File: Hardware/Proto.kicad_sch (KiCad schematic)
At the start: 6 parts, among them J2 Conn_01x04_Male, J3 Conn_01x02_Male, J4 Conn_01x02_Male, J5 Conn_01x02_Male, J6 Conn_01x02_Male, J9 Conn_01x04_MountingPin

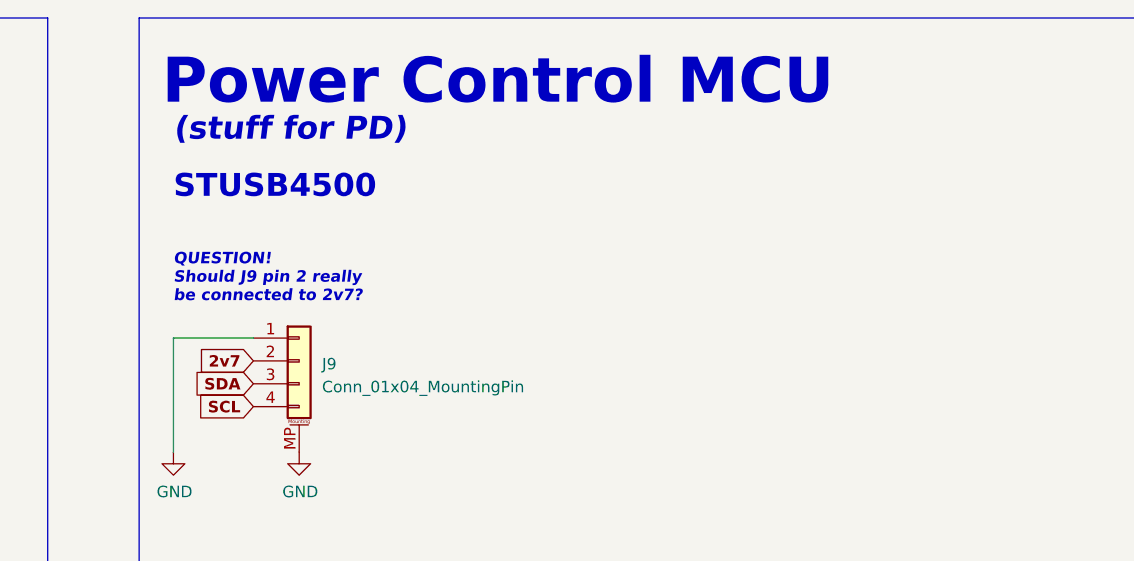
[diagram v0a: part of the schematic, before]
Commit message: .........
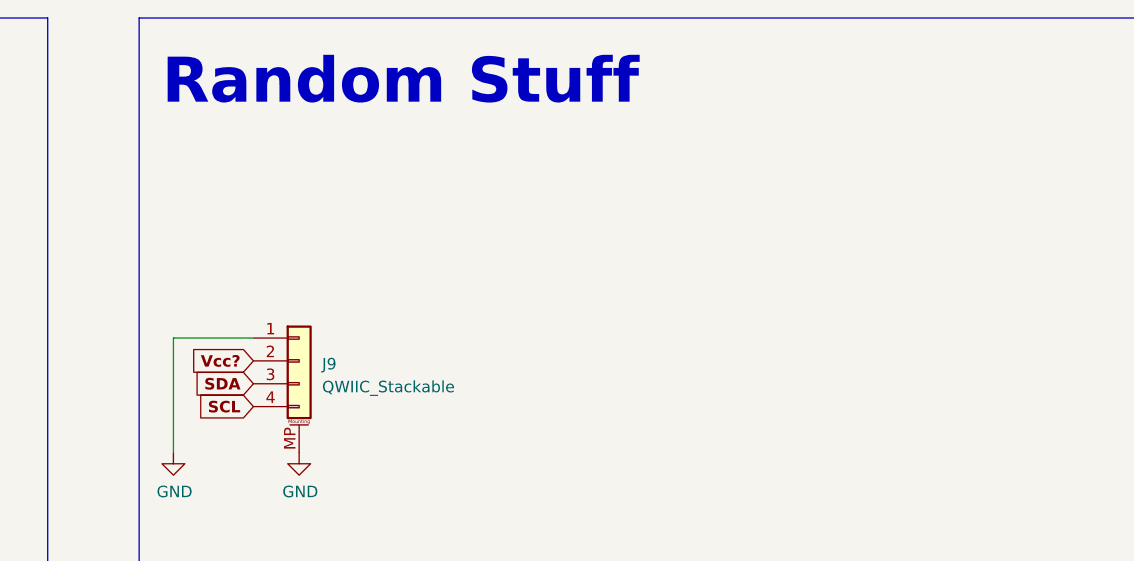
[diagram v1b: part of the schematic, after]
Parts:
- removed J9: Conn_01x04_MountingPin, Tinker:JST_SH_SM04B-SRSS-TB_1x04-1MP_P1.00mm_Horizontal, symbol Connector_Generic_MountingPin:Conn_01x04_MountingPin
- added J9: QWIIC_Stackable, Tinker:QWIIC_Stackable, symbol Connector_QWIIC_Stackable:QWIIC_Stackable
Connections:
- net GND: now also J9.1 (Pin_1), J9.MP (MountPin)
- net SCL: now also J9.4 (Pin_4)
- net SDA: now also J9.3 (Pin_3)
- new net Vcc?: J9.2 (Pin_2)
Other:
- note added: "Random Stuff"
- note removed: "(stuff for PD)"
- note removed: "Power Control MCU"
- note removed: "QUESTION! Should J9 pin 2 really be connected to 2v7?"
- note removed: "STUSB4500"
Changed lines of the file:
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@@
     (effects (font (size 5 5) (thickness 1) bold) (justify left bottom))
-  )
-  (text "QUESTION!\nShould J9 pin 2 really\nbe connected to 2v7?"
-    (at 119.38 45.72 0)
-    (effects (font (size 1.27 1.27) (thickness 0.254) bold italic) (justify left bottom))
-  )
-  (text "STUSB4500" (at 119.38 34.29 180)
-    (effects (font (size 2.54 2.54) (thickness 0.508) bold) (justify left bottom))
   )
   (text "USB" (at 16.51 24.13 0)
     (effects (font (size 5 5) (thickness 1) bold) (justify left bottom))
   )
-  (text "(stuff for PD)" (at 119.38 27.94 0)
-    (effects (font (size 2.54 2.54) (thickness 0.508) bold italic) (justify left bottom))
-  )
-  (text "Power Control MCU" (at 118.11 24.13 0)
+  (text "Random Stuff" (at 118.11 24.13 0)
     (effects (font (size 5 5) (thickness 1) bold) (justify left bottom))
   )
@@
     (effects (font (size 2.54 2.54) (thickness 0.508) bold) (justify left bottom))
   )
-  (global_label "2v7" (shape input) (at 128.27 52.07 180) (fields_autoplaced)
+  (global_label "Vcc?" (shape input) (at 128.27 52.07 180) (fields_autoplaced)
     (effects (font (size 1.27 1.27) (thickness 0.254) bold) (justify right))
-    (property "Intersheet References" "${INTERSHEET_REFS}" (id 0) (at 122.2798 52.197 0)
+    (property "Intersheet References" "${INTERSHEET_REFS}" (id 0) (at 121.3122 51.943 0)
       (effects (font (size 1.27 1.27) (thickness 0.254) bold) (justify right) hide)
     )
@@
     (pin "1")
   )
-  (symbol (lib_id "Connector_Generic_MountingPin:Conn_01x04_MountingPin") (at 133.35 52.07 0) (unit 1)
+  (symbol (lib_id "Connector_QWIIC_Stackable:QWIIC_Stackable") (at 133.35 52.07 0) (unit 1)
     (in_bom yes) (on_board yes) (fields_autoplaced)
     (property "Reference" "J9" (id 0) (at 135.89 52.4255 0)
       (effects (font (size 1.27 1.27)) (justify left))
     )
-    (property "Value" "Conn_01x04_MountingPin" (id 1) (at 135.89 54.9655 0)
+    (property "Value" "QWIIC_Stackable" (id 1) (at 135.89 54.9655 0)
       (effects (font (size 1.27 1.27)) (justify left))
     )
-    (property "Footprint" "Tinker:JST_SH_SM04B-SRSS-TB_1x04-1MP_P1.00mm_Horizontal" (id 2) (at 133.35 52.07 0)
-      (effects (font (size 1.27 1.27)) hide)
+    (property "Footprint" "Tinker:QWIIC_Stackable" (id 2) (at 134.62 62.23 0)
+      (effects (font (size 1.27 1.27)) (justify left) hide)
     )
     (property "Datasheet" "~" (id 3) (at 133.35 52.07 0)
@@
       (reference "J6") (unit 1) (value "Conn_01x02_Male") (footprint "Tinker:PinHeader_1x02_P2.54mm_Vertical")
     )
-    (path "/ae69f442-7b32-4ab2-972d-28d283e0750f"
-      (reference "J9") (unit 1) (value "Conn_01x04_MountingPin") (footprint "Tinker:JST_SH_SM04B-SRSS-TB_1x04-1MP_P1.00mm_Horizontal")
-    )
-  )
+    (path "/b8a785f2-9322-4569-b066-f0e9fc64eafd"
+      (reference "J9") (unit 1) (value "QWIIC_Stackable") (footprint "Tinker:QWIIC_Stackable")
+    )
+  )

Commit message: fiddlin' with stuff...
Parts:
- J2, J3, J4, J5, J6, J9: now left out of the parts list
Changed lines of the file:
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@@
   )
   (symbol (lib_id "Connector:Conn_01x02_Male") (at 33.02 104.14 0) (mirror y) (unit 1)
-    (in_bom yes) (on_board yes)
+    (in_bom no) (on_board yes)
     (property "Reference" "J3" (id 0) (at 32.385 99.06 0))
     (property "Value" "Conn_01x02_Male" (id 1) (at 32.385 101.6 0))
@@
   )
   (symbol (lib_id "Connector:Conn_01x02_Male") (at 58.42 104.14 0) (mirror y) (unit 1)
-    (in_bom yes) (on_board yes)
+    (in_bom no) (on_board yes)
     (property "Reference" "J4" (id 0) (at 57.785 99.06 0))
     (property "Value" "Conn_01x02_Male" (id 1) (at 57.785 101.6 0))
@@
   )
   (symbol (lib_id "Connector_QWIIC_Stackable:QWIIC_Stackable") (at 133.35 52.07 0) (unit 1)
-    (in_bom yes) (on_board yes) (fields_autoplaced)
+    (in_bom no) (on_board yes) (fields_autoplaced)
     (property "Reference" "J9" (id 0) (at 135.89 52.4255 0)
       (effects (font (size 1.27 1.27)) (justify left))
@@
   )
   (symbol (lib_id "Connector:Conn_01x02_Male") (at 58.42 148.59 0) (mirror y) (unit 1)
-    (in_bom yes) (on_board yes)
+    (in_bom no) (on_board yes)
     (property "Reference" "J6" (id 0) (at 57.15 143.51 0)
       (effects (font (size 1.27 1.27)) (justify right))
@@
   )
   (symbol (lib_id "Connector:Conn_01x04_Male") (at 31.75 34.29 0) (mirror y) (unit 1)
-    (in_bom yes) (on_board yes)
+    (in_bom no) (on_board yes)
     (property "Reference" "J2" (id 0) (at 27.94 26.67 0)
       (effects (font (size 1.27 1.27)) (justify right))
@@
   )
   (symbol (lib_id "Connector:Conn_01x02_Male") (at 33.02 148.59 0) (mirror y) (unit 1)
-    (in_bom yes) (on_board yes) (fields_autoplaced)
+    (in_bom no) (on_board yes) (fields_autoplaced)
     (property "Reference" "J5" (id 0) (at 32.385 143.51 0))
     (property "Value" "Conn_01x02_Male" (id 1) (at 32.385 146.05 0))
